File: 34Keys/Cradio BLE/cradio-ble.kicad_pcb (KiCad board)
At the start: 2 copper layers, 108.7 x 85.2 mm, 19 parts, among them SW10 SW_PUSH, SW11 SW_PUSH, SW12 SW_PUSH, SW14 SW_PUSH, SW15 SW_PUSH, SW16 SW_PUSH, SW17 SW_PUSH, SW18 SW_PUSH, SW2 SW_PUSH, SW20 SW_PUSH, SW21 SW_PUSH, SW3 SW_PUSH, SW4 SW_PUSH, SW5 SW_PUSH, SW6 SW_PUSH, SW8 SW_PUSH, SW9 SW_PUSH, U1 ProMicro

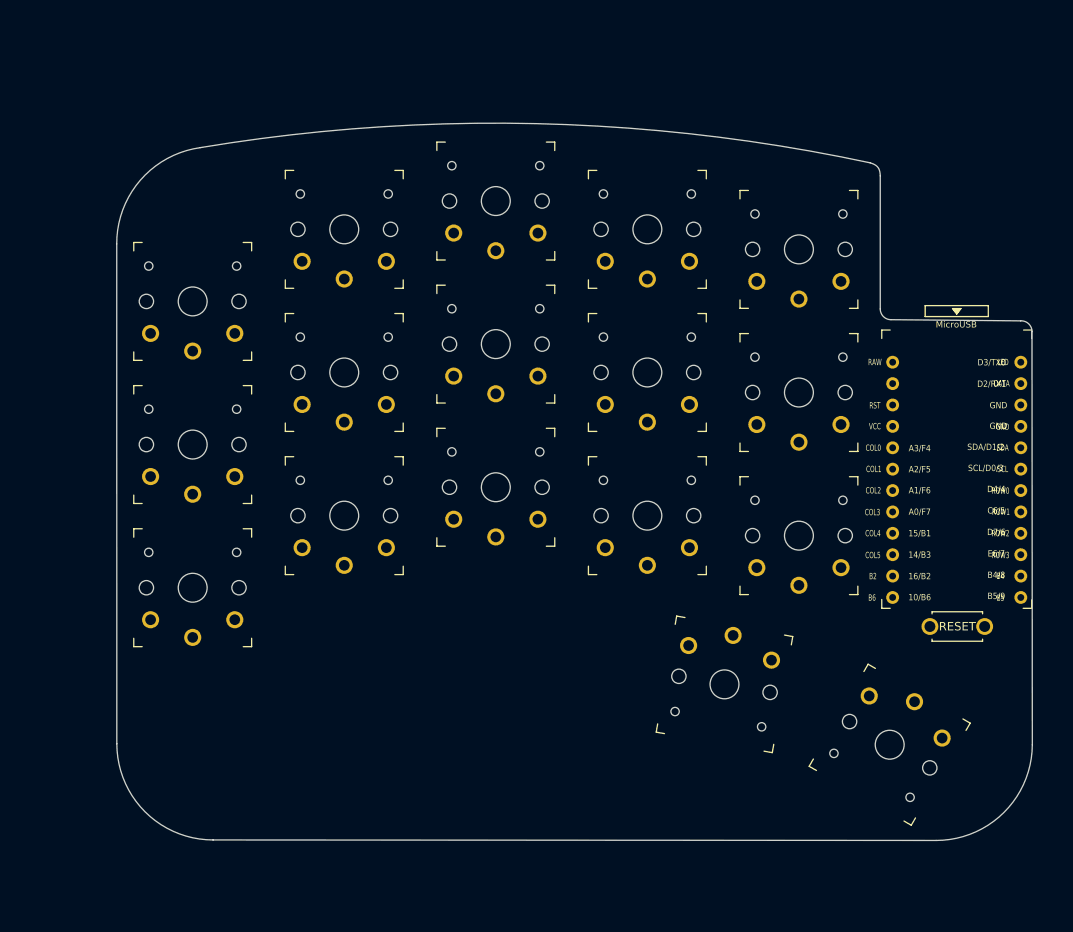
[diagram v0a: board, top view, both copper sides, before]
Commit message: Add files via upload
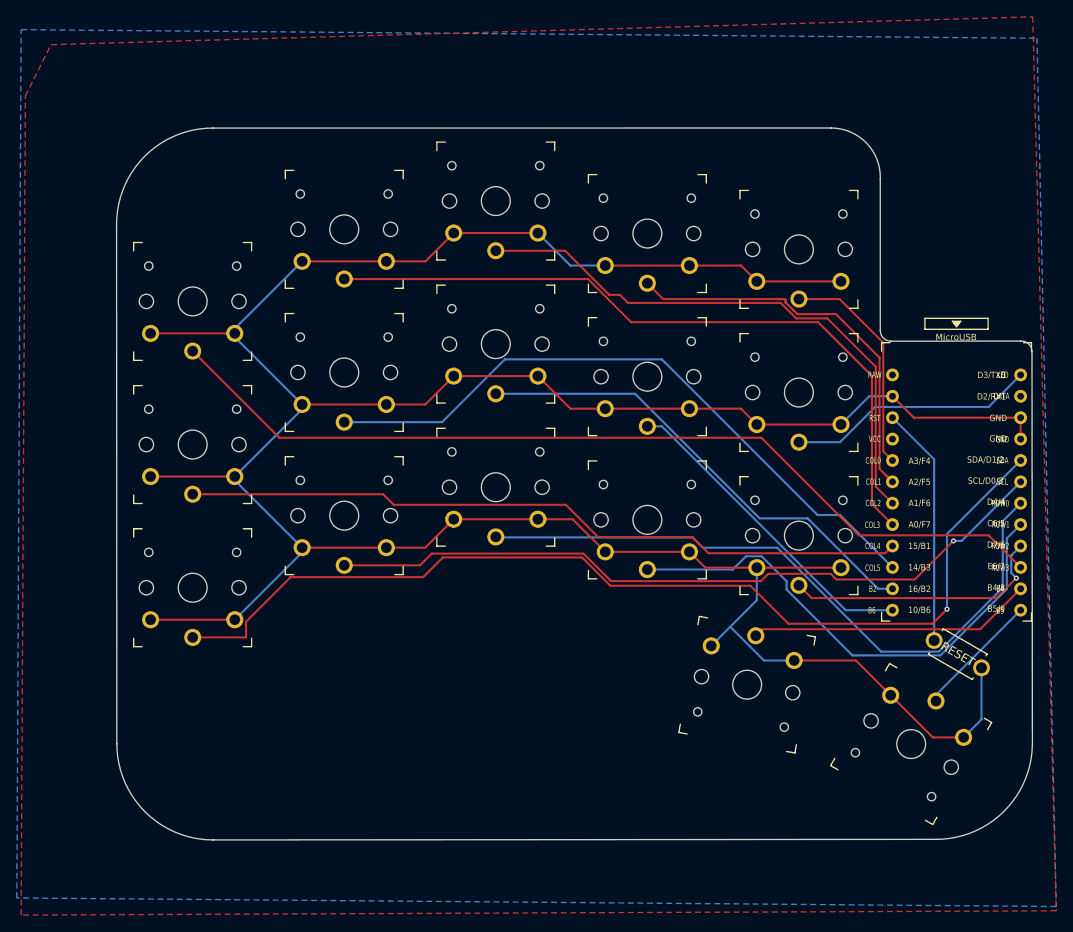
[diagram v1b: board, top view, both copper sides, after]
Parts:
- moved RSW1 3.28 mm to (134.9, 79.0), turned to 150 degrees
- moved SW20 2.69 mm to (109.8, 82.6)
- moved SW21 2.55 mm to (129.3, 89.7)
- moved U1 1.51 mm to (134.7, 60.3)
- moved SW11 0.50 mm to (98.0, 46.0)
- moved SW17 0.50 mm to (98.0, 63.0)
- moved SW5 0.50 mm to (98.0, 29.0)
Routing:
- net GND: track 0.00 -> 372.6 mm
- net SDA: track 0.00 -> 119.9 mm, vias 0 -> 1
- net row3: track 0.00 -> 109.0 mm
- net SCL: track 0.00 -> 87.7 mm, vias 0 -> 1
- net col4: track 0.00 -> 86.4 mm
- net col3: track 0.00 -> 86.1 mm
- net row0: track 0.00 -> 79.9 mm
- net col5: track 0.00 -> 78.4 mm
- net col2: track 0.00 -> 68.3 mm
- net row1: track 0.00 -> 60.4 mm
- net Net-(U1-Pad14): track 0.00 -> 56.7 mm
- net col1: track 0.00 -> 49.1 mm
- net Net-(U1-Pad13): track 0.00 -> 38.2 mm
- net Net-(U1-Pad11): track 0.00 -> 33.8 mm
- net row2: track 0.00 -> 32.0 mm, vias 0 -> 1
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- added copper zone on B.Cu, net (none)
- added copper zone on F.Cu, net (none)
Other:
- board size 108.7 x 85.2 mm -> 108.8 x 84.6 mm
